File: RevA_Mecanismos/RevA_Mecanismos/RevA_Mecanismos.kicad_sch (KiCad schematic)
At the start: 26 parts, among them J1 PROG, SW1 SW_Push, U1 STM32L431RCTx, Y1 16MHz

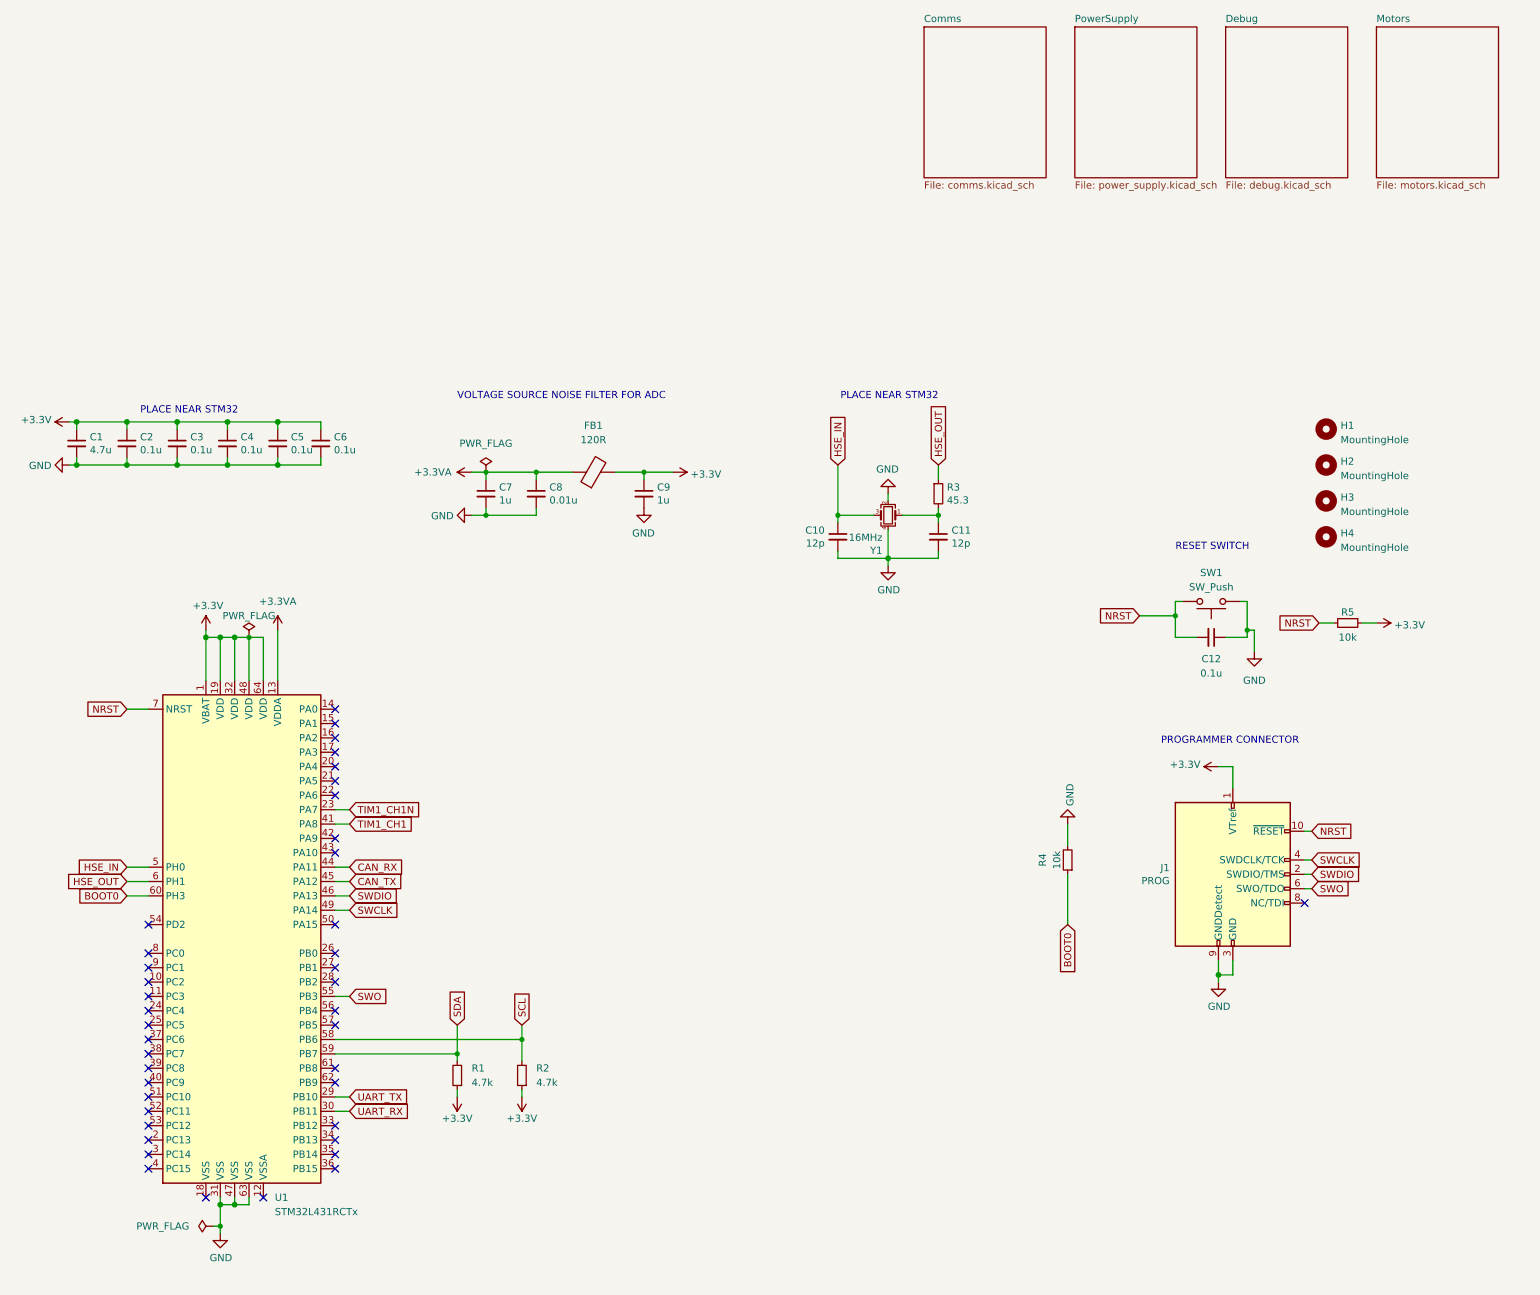
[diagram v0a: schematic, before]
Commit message: Created PCB project
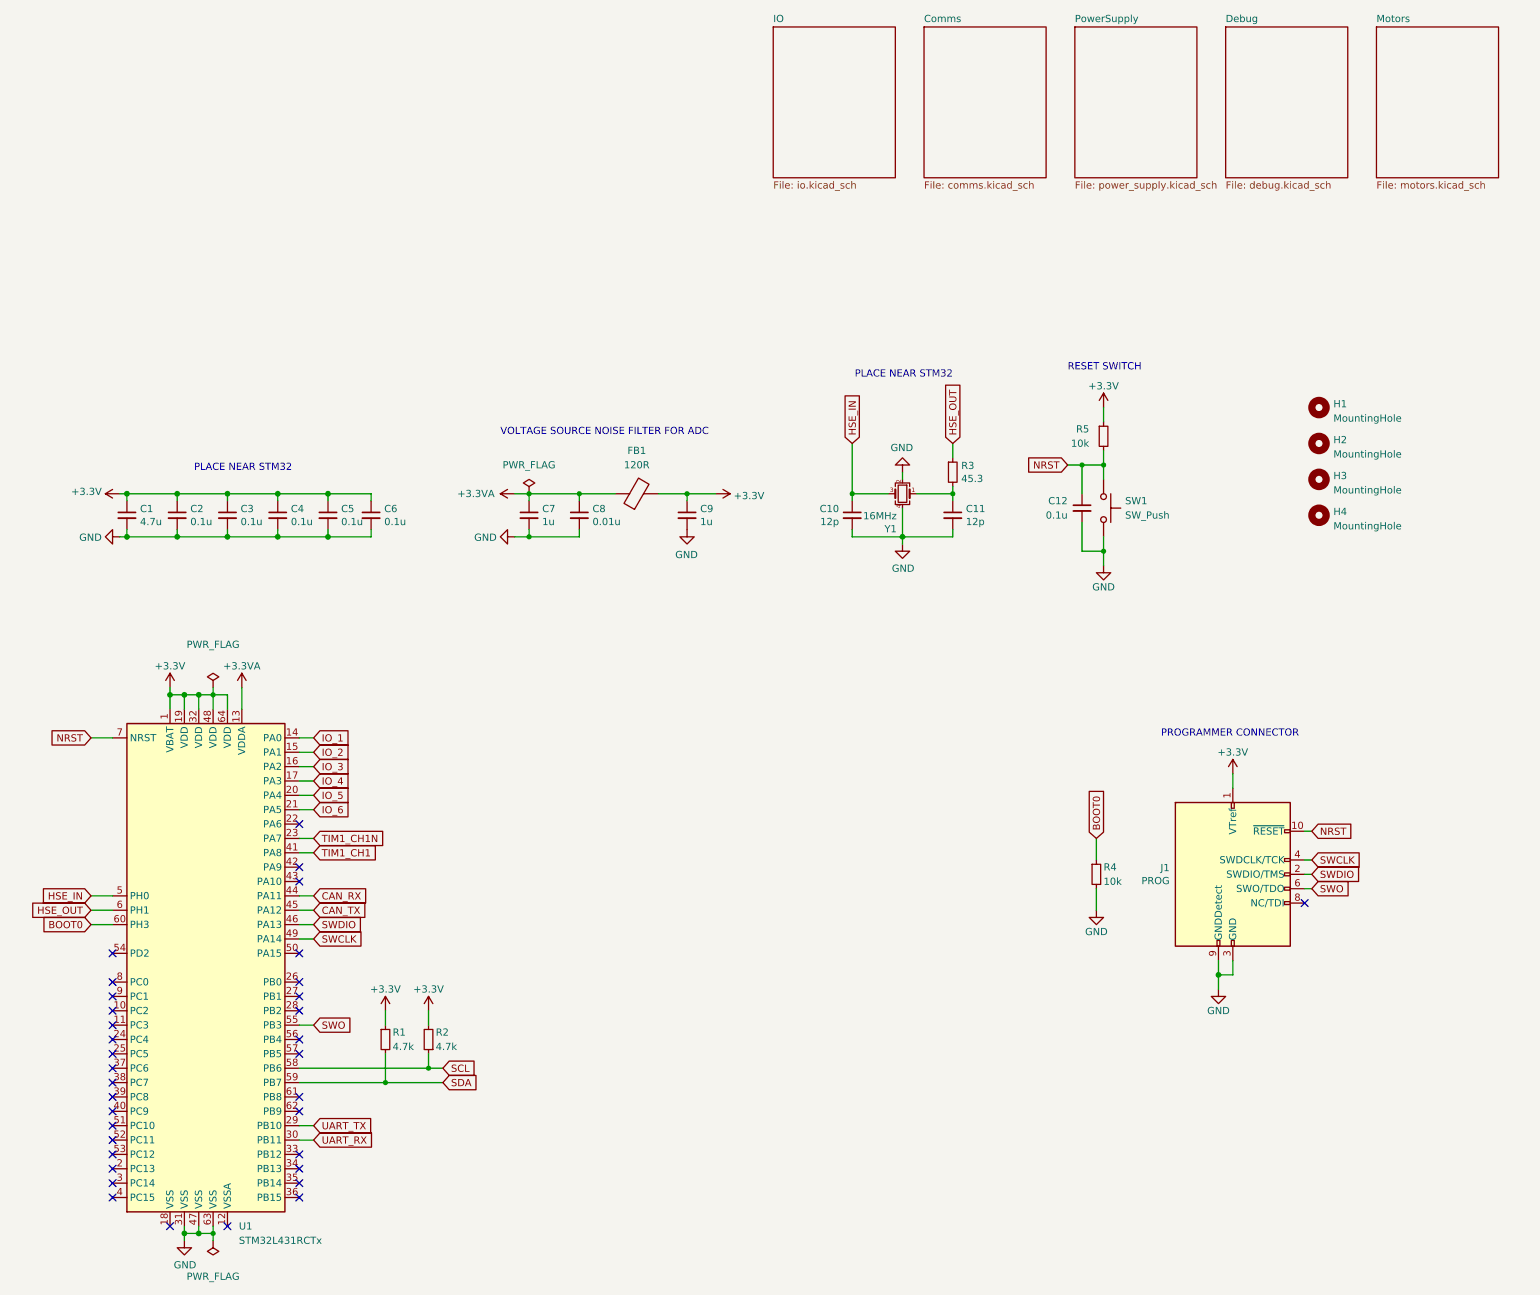
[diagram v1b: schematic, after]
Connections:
- net +3.3V: now also R2.2; no longer R2.1
- net GND: now also C12.2, SW1.2; no longer C12.1, SW1.1
- net NRST: now also C12.1, SW1.1; no longer C12.2, SW1.2
- net SCL: now also R2.1; no longer R2.2
- net IO_1: now reaches U1.14 (PA0)
- net IO_2: now reaches U1.15 (PA1)
- net IO_3: now reaches U1.16 (PA2)
- net IO_4: now reaches U1.17 (PA3)
- net IO_5: now reaches U1.20 (PA4)
- net IO_6: now reaches U1.21 (PA5)
- no-connect marks 41 -> 35
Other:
- added sheet IO (io.kicad_sch)
- moved on the sheet: C1, C10, C11, C12, C2, C3, C4, C5, C6, C7, C8, C9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
